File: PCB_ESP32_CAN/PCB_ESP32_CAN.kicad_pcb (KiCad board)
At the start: 2 copper layers, 52.2 x 67.2 mm, 53 parts, among them J1 USB_C_Receptacle_USB2.0, J2 CAN, J3 CAN, J4 CAN, J5 CAN, Q1 Q_NPN_BCE, Q2 Q_NPN_BCE, U1 ESP32-WROOM-32, U2 CP2102N-A01-GQFN24, U3 SN65HVD232, U4 NCP1117-3.3_SOT223

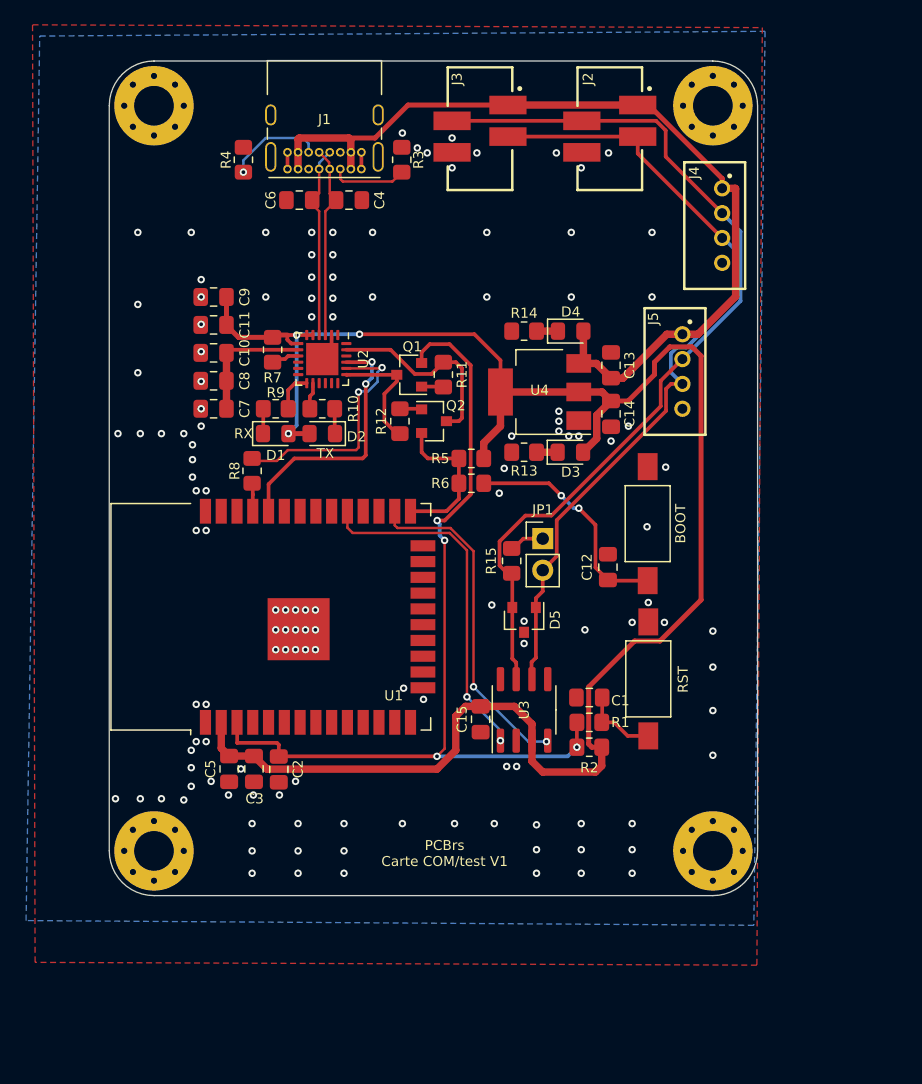
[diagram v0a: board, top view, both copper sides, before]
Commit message: regime sur la carte esp32
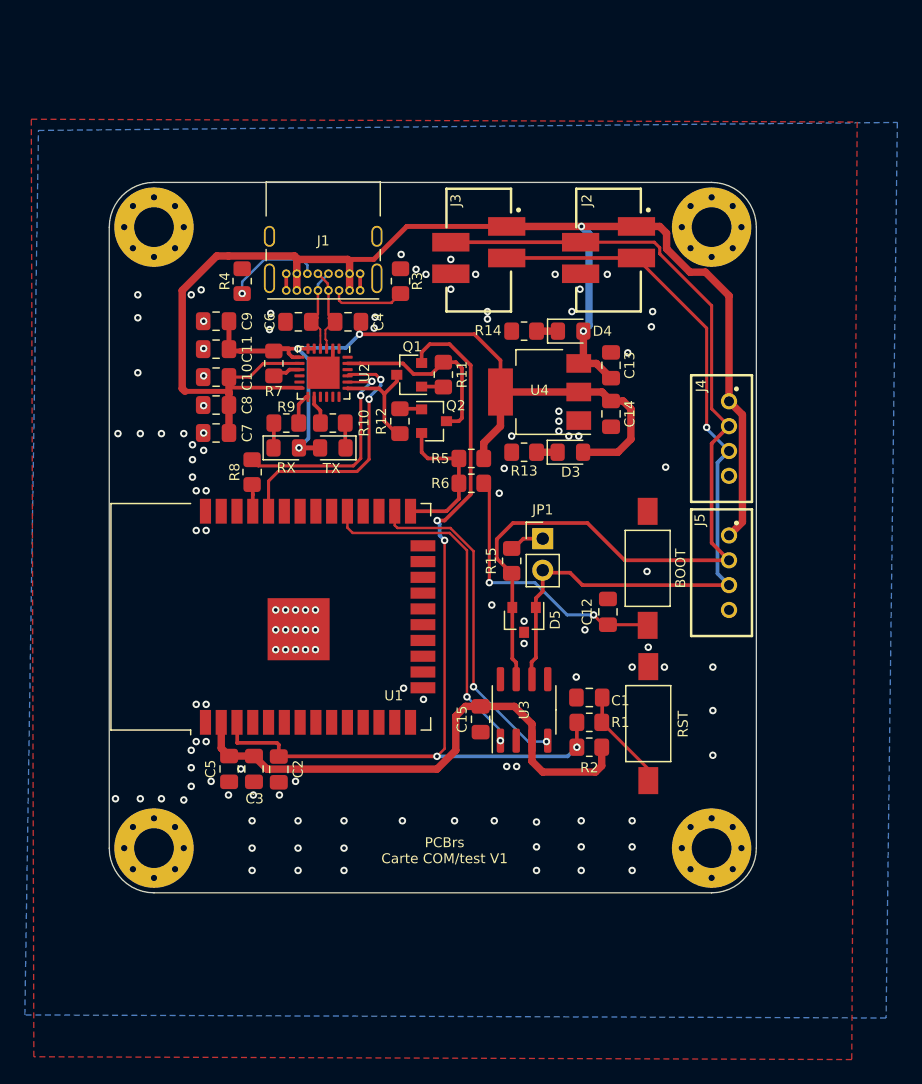
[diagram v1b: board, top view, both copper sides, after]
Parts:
- moved J4 17.2 mm to (101.9, 90.4)
- moved J5 16.6 mm to (101.9, 101.2)
- moved C4 9.80 mm to (71.8, 81.0)
- moved C6 9.80 mm to (67.8, 81.0)
- moved H3 9.78 mm to (101.1, 73.4)
- moved J1 9.78 mm to (72.8, 78.5)
- moved J2 9.78 mm to (92.8, 75.2)
- moved J3 9.78 mm to (82.4, 75.2)
- moved R3 9.78 mm to (76.0, 77.7)
- moved R4 9.78 mm to (63.3, 77.7)
- moved H1 9.77 mm to (56.2, 73.4)
- moved BOOT 3.60 mm to (96.0, 100.8)
- moved C12 3.60 mm to (92.8, 104.3)
- moved RST 3.60 mm to (96.0, 113.3)
- moved C10 1.96 mm to (61.2, 85.5)
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- renumbered D1 to RX, D2 to TX
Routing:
- net +3V3: track 151.4 -> 108.1 mm
- net +5V: track 82.3 -> 112.2 mm, vias 0 -> 2
- net /USB+: track 15.8 -> 7.93 mm
- net /USB-: track 15.5 -> 7.76 mm
- net Net-(U2-Pad12): track 0.00 -> 5.52 mm
- net Net-(C12-Pad1): track 18.5 -> 22.4 mm
- net /CANH: track 74.7 -> 78.0 mm
- net Net-(C1-Pad1): track 6.22 -> 8.26 mm
- net Net-(R8-Pad2): track 19.7 -> 17.8 mm
- net /RTS: track 9.88 -> 8.96 mm
- net Net-(R9-Pad2): track 3.23 -> 2.50 mm
- net /CANL: track 66.0 -> 65.3 mm, vias 0 -> 1
- net /DTR: track 16.1 -> 15.5 mm
- net GND: vias 131 -> 119
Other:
- board size 52.2 x 67.2 mm -> 52.1 x 57.2 mm
- board text removed: "RX"
- board text removed: "TX"
